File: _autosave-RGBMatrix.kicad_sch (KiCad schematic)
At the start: 239 parts, among them Q17 PNP, Q18 PNP, Q19 PNP, Q20 PNP, Q21 PNP, Q22 PNP, Q23 PNP, Q24 PNP, Q25 PNP, Q26 PNP, Q27 PNP, Q28 PNP, Q29 PNP, Q30 PNP, Q31 PNP, Q32 PNP, U1 74LS596, U2 74LS596, U3 74LS596, U4 74LS596, U5 74LS596, U6 74LS596, U7 74154

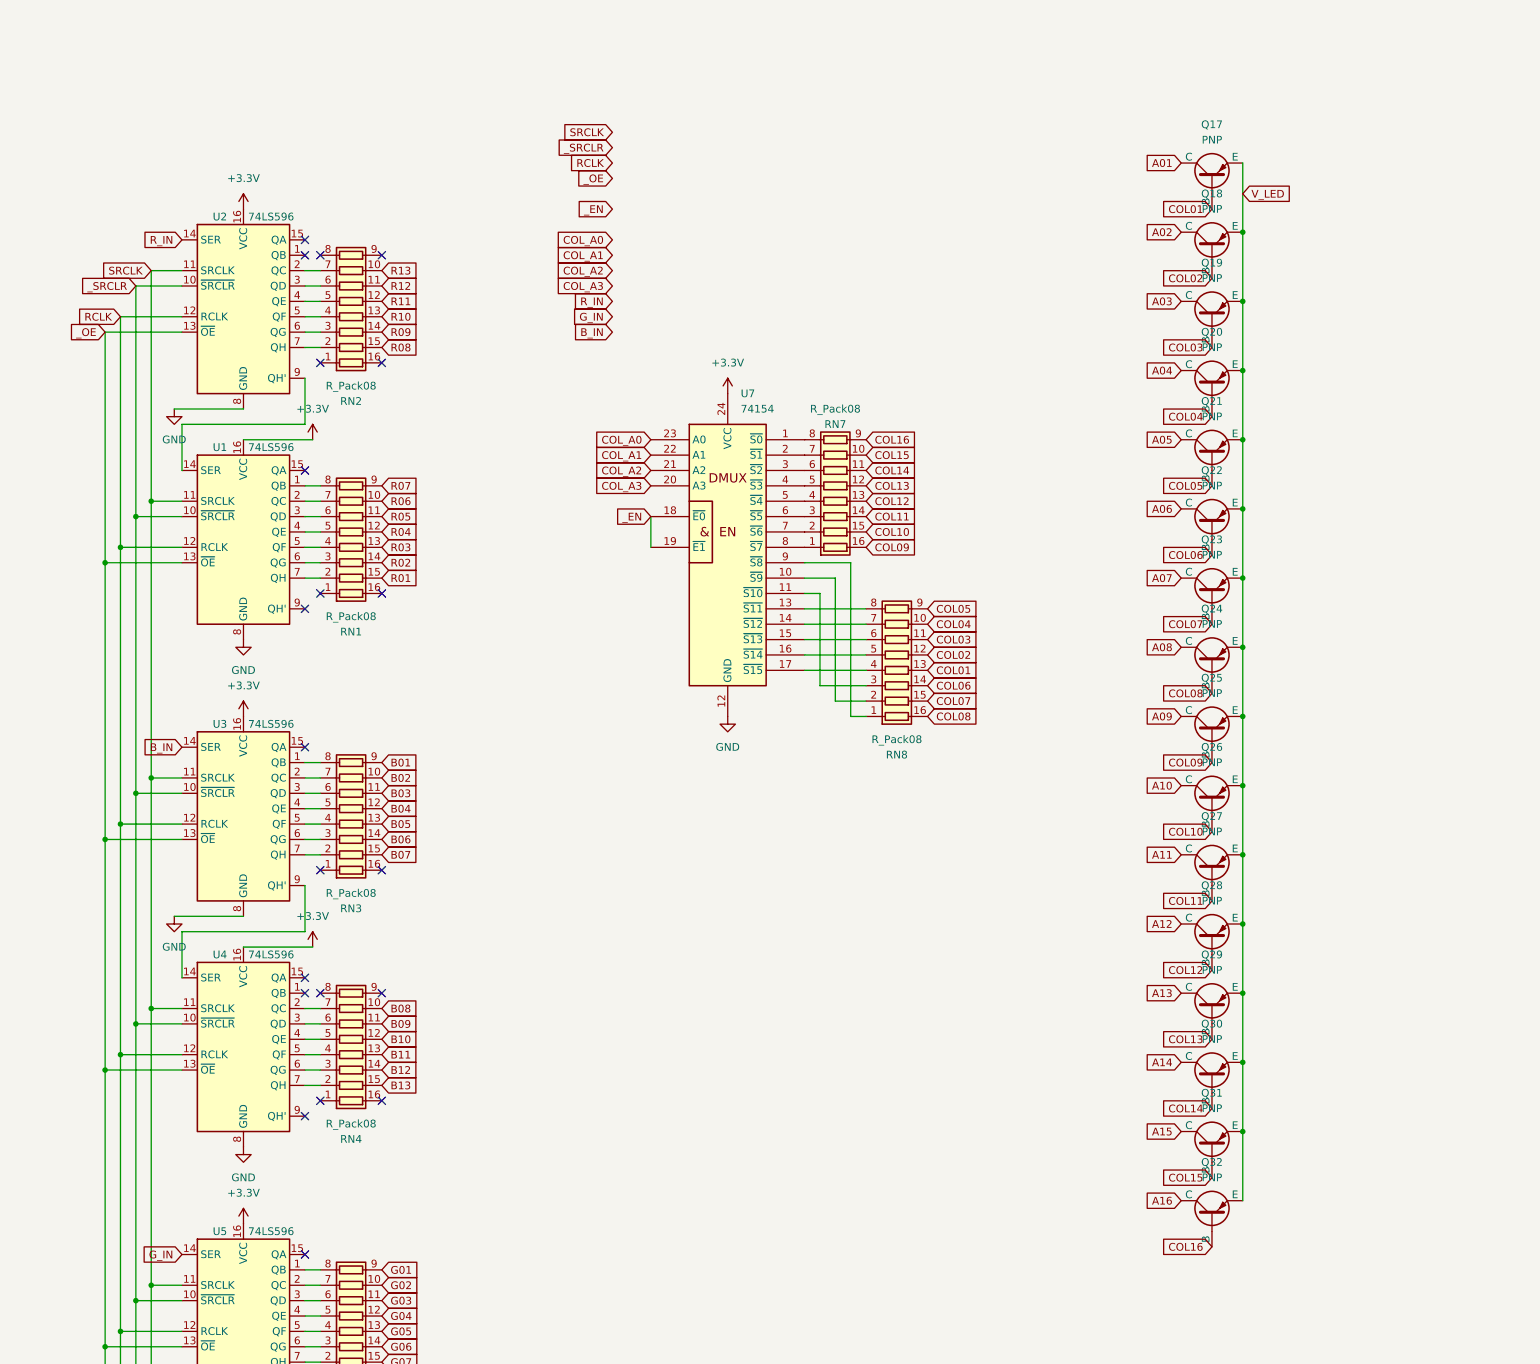
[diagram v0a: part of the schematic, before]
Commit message: update
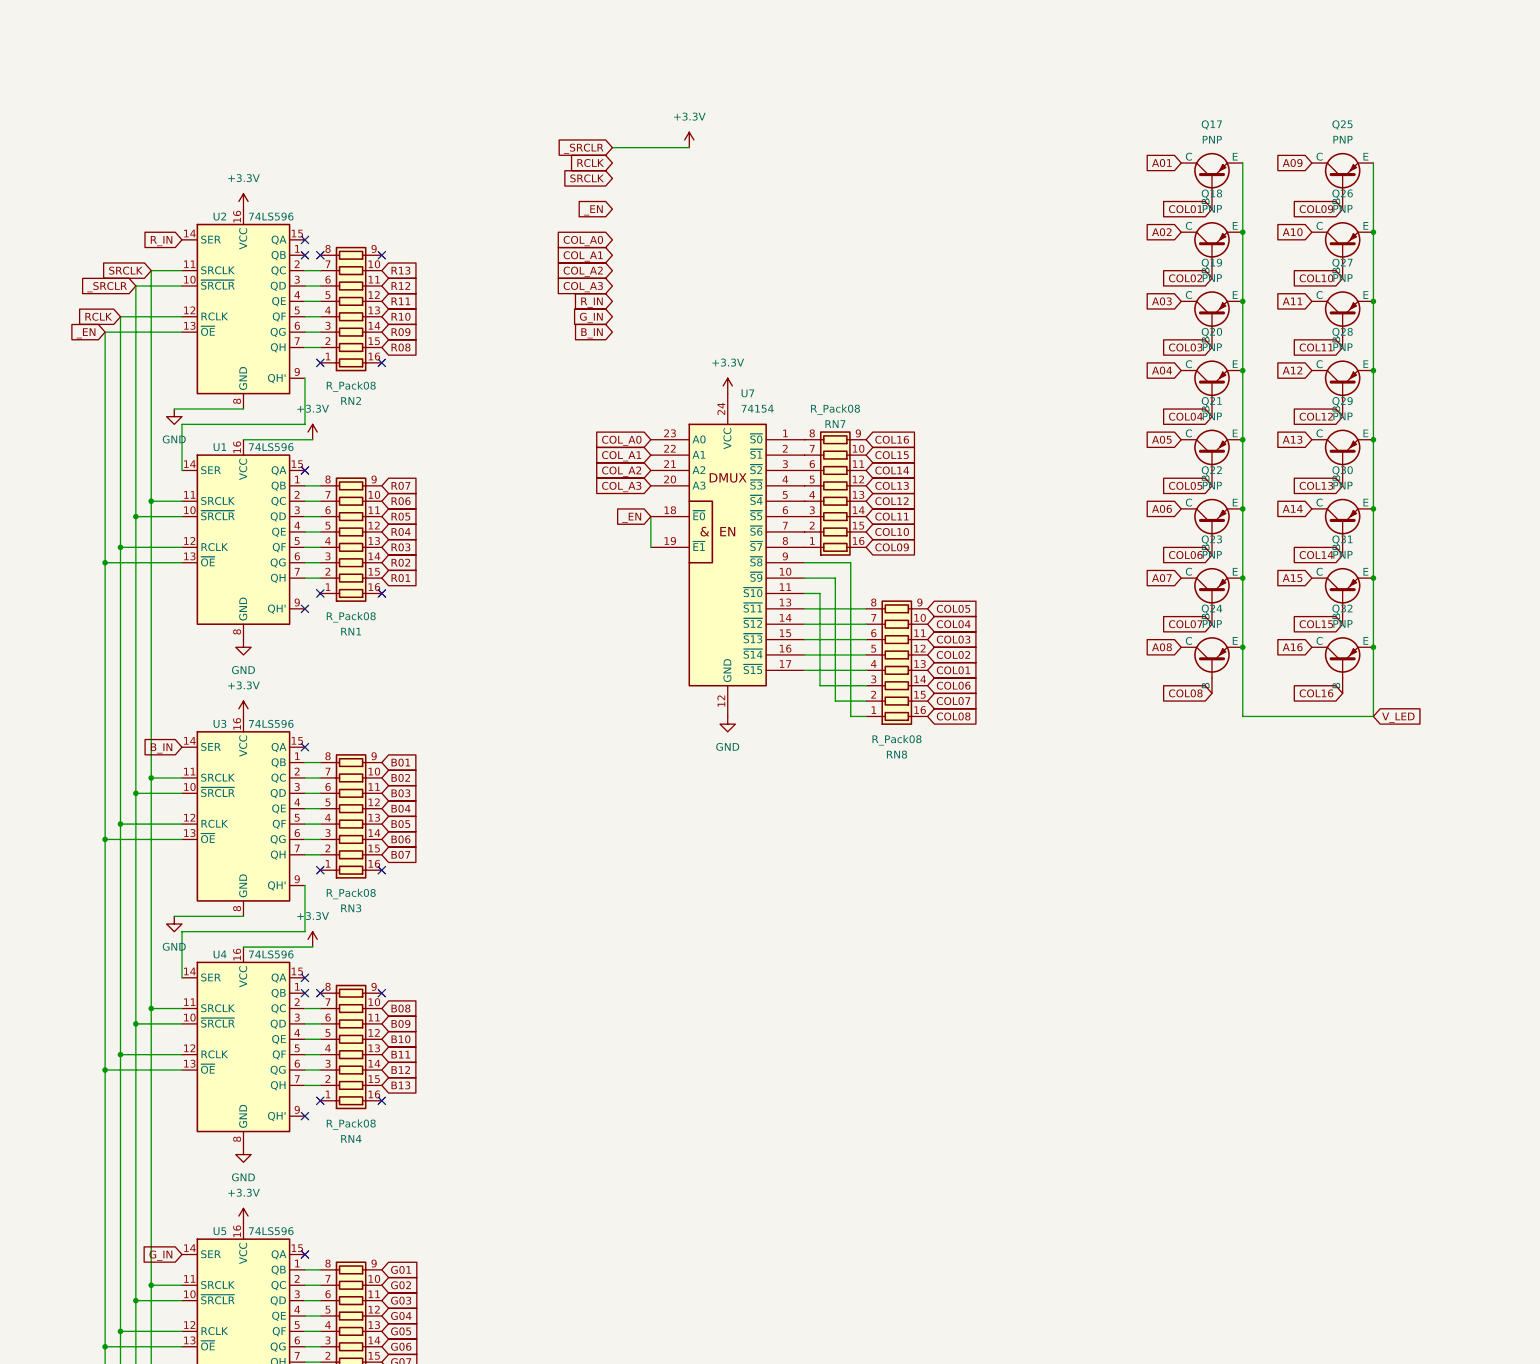
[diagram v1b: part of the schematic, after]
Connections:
- net _OE is gone; now on net _EN: U1.13 (~{OE}), U2.13 (~{OE}), U3.13 (~{OE}), U4.13 (~{OE}), U5.13 (~{OE}), U6.13 (~{OE})
- net _SRCLR is gone; now on net +3.3V: U1.10 (~{SRCLR}), U2.10 (~{SRCLR}), U3.10 (~{SRCLR}), U4.10 (~{SRCLR}), U5.10 (~{SRCLR}), U6.10 (~{SRCLR})
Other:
- moved on the sheet: Q25, Q26, Q27, Q28, Q29, Q30, Q31, Q32
